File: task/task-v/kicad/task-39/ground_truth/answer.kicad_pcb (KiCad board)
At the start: 4 copper layers, 160 x 160 mm, 1 part, among them U1 BGA-225

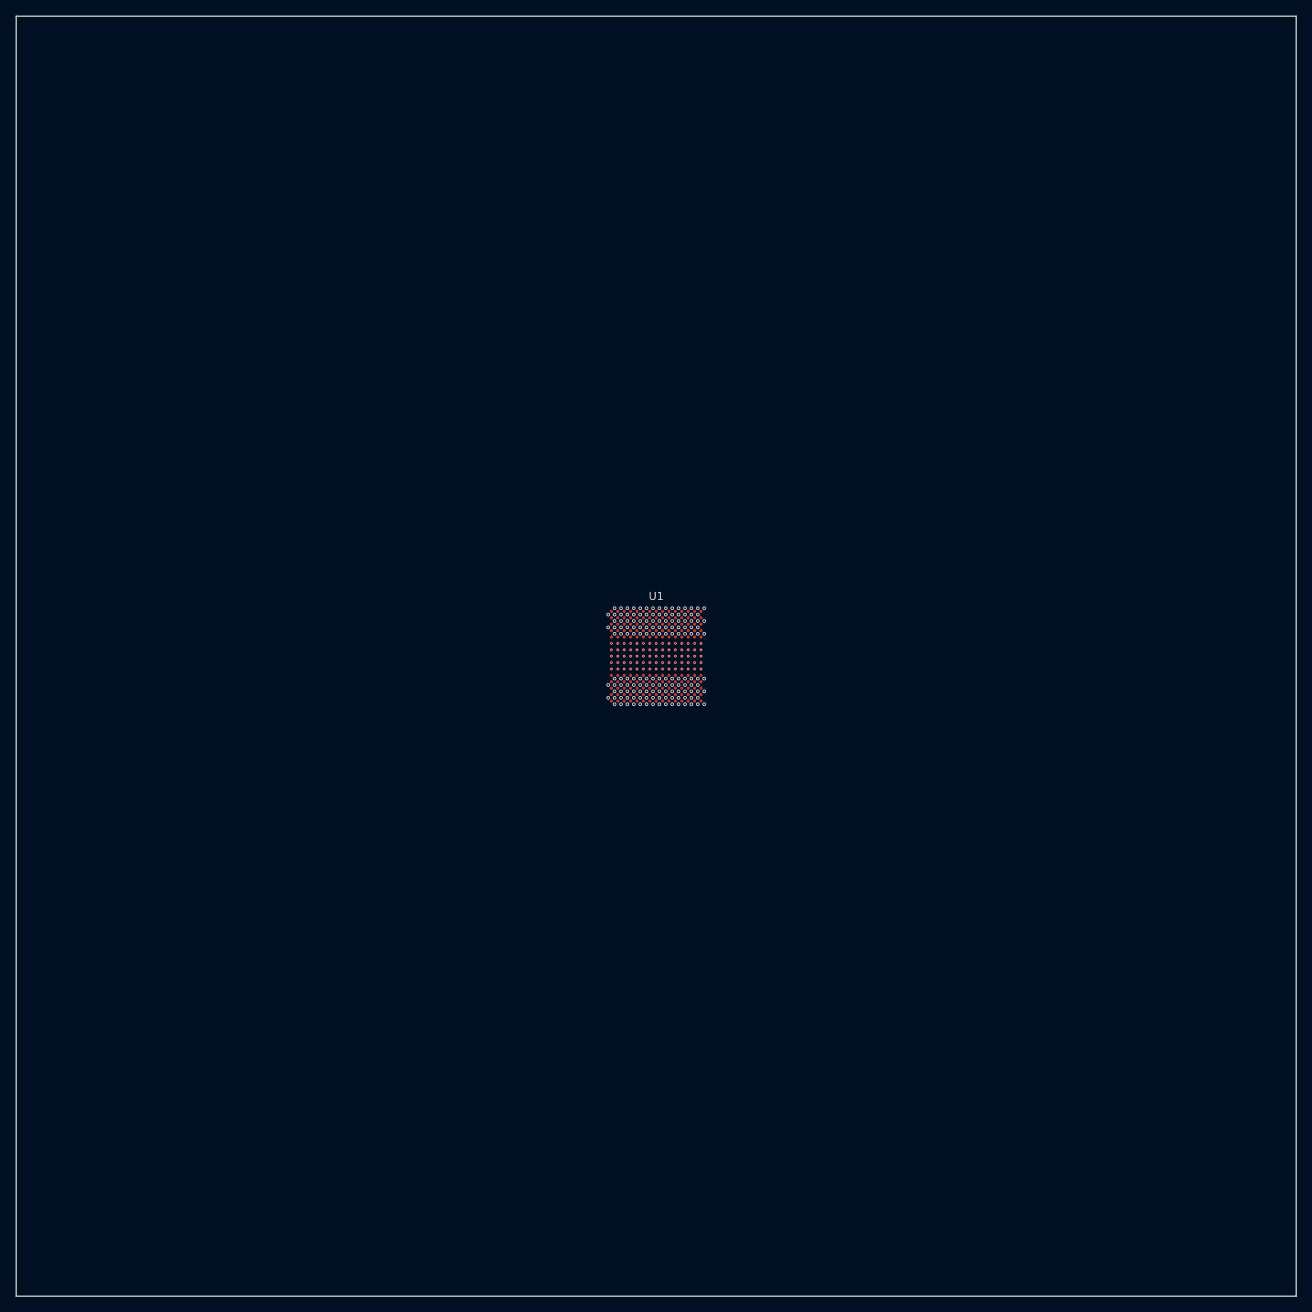
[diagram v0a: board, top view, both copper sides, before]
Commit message: Refine engineering task metadata and instructions
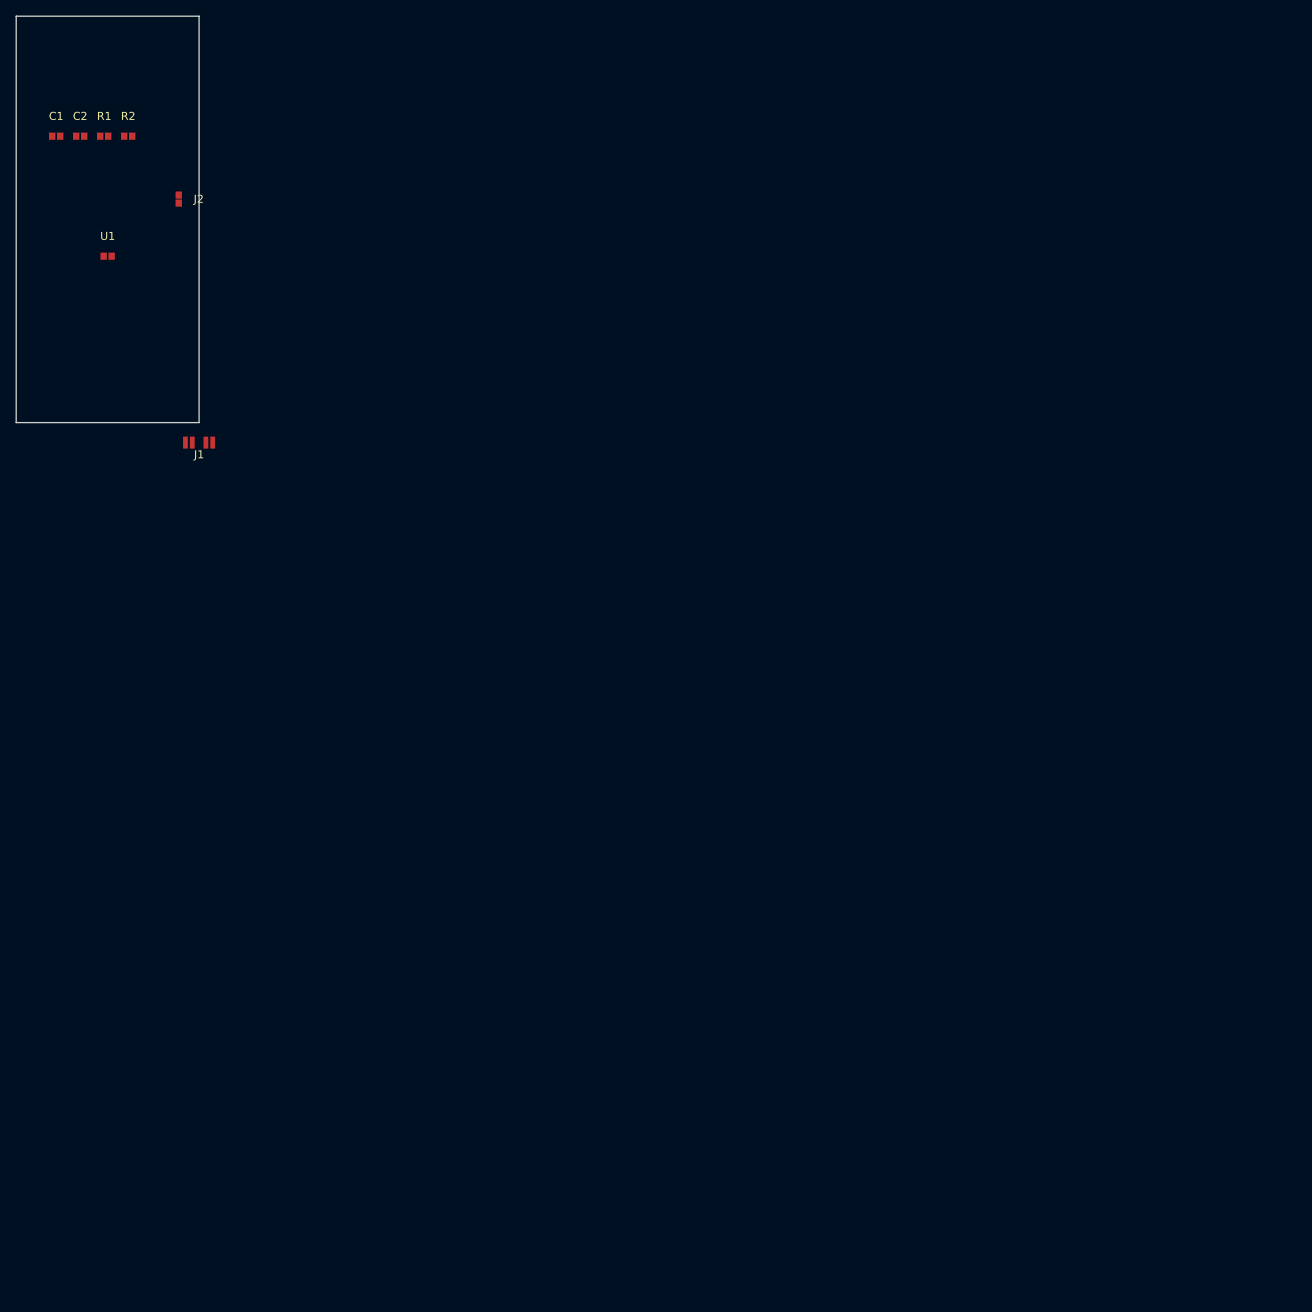
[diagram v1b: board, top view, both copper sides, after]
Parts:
- added C1: C1, Capacitor_SMD:C_0402_1005Metric, F.Cu at (5.00, 15.0)
- added C2: C2, Capacitor_SMD:C_0402_1005Metric, F.Cu at (8.00, 15.0)
- added J1: USB_C_Receptacle, Connector_USB:USB_C_Receptacle_GCT_USB4105-GF-A, F.Cu at (22.9, 50.8)
- added J2: J2, Connector_PinSocket_2.54mm:PinSocket_1x16_P2.54mm_Vertical, F.Cu at (20.3, 22.9)
- added R1: R1, Resistor_SMD:R_0402_1005Metric, F.Cu at (11.0, 15.0)
- added R2: R2, Resistor_SMD:R_0402_1005Metric, F.Cu at (14.0, 15.0)
- U1: value BGA-225 -> U1; footprint Package_BGA:BGA-225_15x15_P0.8mm -> Package_QFP:LQFP-48_7x7mm_P0.5mm
- moved U1 84.9 mm to (11.4, 30.0)
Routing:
- net (no net): vias 225 -> 0
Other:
- board size 160 x 160 mm -> 22.9 x 50.8 mm
- copper layers 4 -> 2
